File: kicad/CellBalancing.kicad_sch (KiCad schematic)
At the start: 10 parts, among them U15 ETA3000

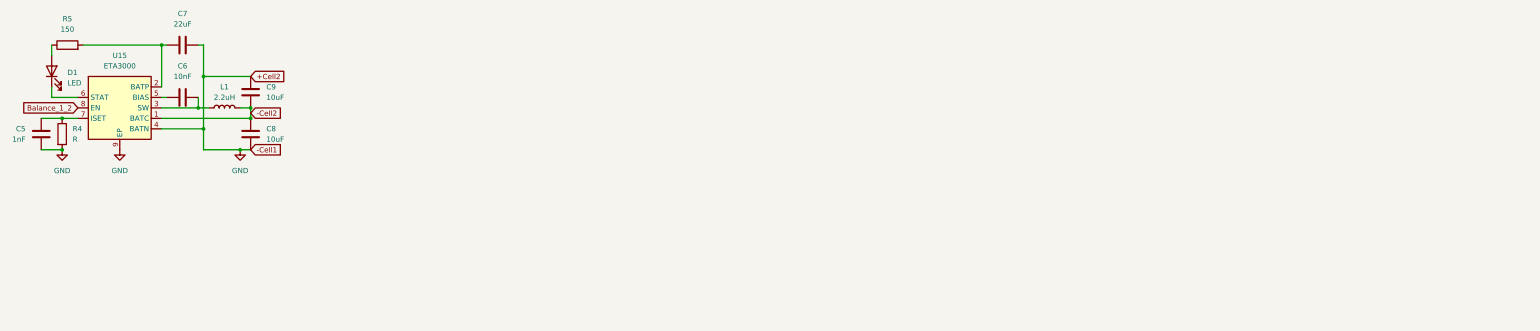
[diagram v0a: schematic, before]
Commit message: .gitignore
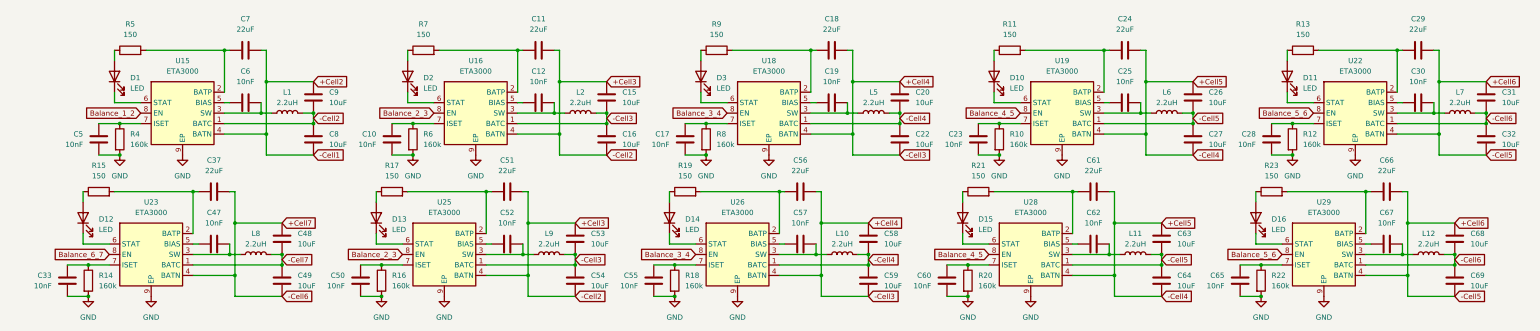
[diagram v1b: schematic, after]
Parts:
- added C10, C12, C17, C19, C23, C25, C28, C30, C33, C47, C50, C52, C55, C57, C60, C62, C65, C67: 10nF, symbol Device:C
- added C11, C18, C24, C29, C37, C51, C56, C61, C66: 22uF, symbol Device:C
- added C15, C16, C20, C22, C26, C27, C31, C32, C48, C49, C53, C54, C58, C59, C63, C64, C68, C69: 10uF, symbol Device:C
- added D10, D11, D12, D13, D14, D15, D16, D2, D3: LED, symbol Device:LED
- added L10, L11, L12, L2, L5, L6, L7, L8, L9: 2.2uH, symbol Device:L
- added R10, R12, R14, R16, R18, R20, R22, R6, R8: 160k, symbol Device:R
- added R11, R13, R15, R17, R19, R21, R23, R7, R9: 150, symbol Device:R
- added U16, U18, U19, U22, U23, U25, U26, U28, U29: ETA3000, Package_DFN_QFN:DFN-8-1EP_2x2mm_P0.5mm_EP0.9x1.3mm, symbol Battery_Management:ETA3000
- C5: value 1nF -> 10nF
- R4: value R -> 160k
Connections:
- net GND: now also C10.2, C17.2, C23.2, C28.2, C33.2, C50.2, C55.2, C60.2, C65.2, R10.2, R12.2, R14.2, R16.2, R18.2, R20.2, R22.2, R6.2, R8.2, U16.9 (EP), U18.9 (EP), U19.9 (EP), U22.9 (EP), U23.9 (EP), U25.9 (EP), U26.9 (EP), U28.9 (EP), U29.9 (EP); no longer C7.2, C8.2, C9.1, U15.4 (BATN)
- net -Cell2 renamed +Cell3
- net +Cell3: now also C11.2, C15.1, C16.2, C51.2, C53.1, C54.2, U16.4 (BATN), U25.4 (BATN)
- new net: D16.2 (A), R23.1
- new net: C66.1, R23.2, U29.2 (BATP)
- new net: C52.1, U25.5 (BIAS)
- new net: C52.2, L9.1, U25.3 (SW)
- new net: C51.1, R17.2, U25.2 (BATP)
- new net: D13.1 (K), U25.6 (STAT)
- new net: C50.1, R16.1, U25.7 (ISET)
- new net: D15.2 (A), R21.1
- new net: C61.1, R21.2, U28.2 (BATP)
- new net: D2.1 (K), U16.6 (STAT)
- new net: D2.2 (A), R7.1
- new net: D16.1 (K), U29.6 (STAT)
- new net: C18.1, R9.2, U18.2 (BATP)
- new net: C19.2, L5.1, U18.3 (SW)
- new net: C19.1, U18.5 (BIAS)
- new net: D3.1 (K), U18.6 (STAT)
- new net: C17.1, R8.1, U18.7 (ISET)
- new net: D15.1 (K), U28.6 (STAT)
- new net: C30.1, U22.5 (BIAS)
- new net: C30.2, L7.1, U22.3 (SW)
- new net: D12.1 (K), U23.6 (STAT)
- new net: D12.2 (A), R15.1
- new net: C65.1, R22.1, U29.7 (ISET)
- new net: C47.1, U23.5 (BIAS)
- new net: C47.2, L8.1, U23.3 (SW)
- new net: C56.1, R19.2, U26.2 (BATP)
- new net: C24.1, R11.2, U19.2 (BATP)
- new net: C60.1, R20.1, U28.7 (ISET)
- new net: C62.2, L11.1, U28.3 (SW)
- new net: C11.1, R7.2, U16.2 (BATP)
- new net: C12.2, L2.1, U16.3 (SW)
- new net: C12.1, U16.5 (BIAS)
- new net: C10.1, R6.1, U16.7 (ISET)
- new net: D14.1 (K), U26.6 (STAT)
- new net: D14.2 (A), R19.1
- new net: C57.2, L10.1, U26.3 (SW)
- new net: D13.2 (A), R17.1
- new net: C33.1, R14.1, U23.7 (ISET)
- new net: D11.1 (K), U22.6 (STAT)
- new net: D11.2 (A), R13.1
- new net: C37.1, R15.2, U23.2 (BATP)
- new net: C67.1, U29.5 (BIAS)
- new net: C67.2, L12.1, U29.3 (SW)
- new net: C29.1, R13.2, U22.2 (BATP)
- new net: C28.1, R12.1, U22.7 (ISET)
- new net: C57.1, U26.5 (BIAS)
- new net: C55.1, R18.1, U26.7 (ISET)
- new net: D3.2 (A), R9.1
- new net: C25.2, L6.1, U19.3 (SW)
- new net: C25.1, U19.5 (BIAS)
- new net: D10.1 (K), U19.6 (STAT)
- new net: C23.1, R10.1, U19.7 (ISET)
- new net: C62.1, U28.5 (BIAS)
- new net: D10.2 (A), R11.1
- new net +Cell2: C7.2, C8.2, C9.1, U15.4 (BATN)
- new net +Cell4: C15.2, C16.1, C18.2, C20.1, C22.2, C53.2, C54.1, C56.2, C58.1, C59.2, L2.2, L9.2, U16.1 (BATC), U18.4 (BATN), U25.1 (BATC), U26.4 (BATN)
- new net +Cell5: C20.2, C22.1, C24.2, C26.1, C27.2, C58.2, C59.1, C61.2, C63.1, C64.2, L10.2, L5.2, U18.1 (BATC), U19.4 (BATN), U26.1 (BATC), U28.4 (BATN)
- new net +Cell6: C26.2, C27.1, C29.2, C31.1, C32.2, C63.2, C64.1, C66.2, C68.1, C69.2, L11.2, L6.2, U19.1 (BATC), U22.4 (BATN), U28.1 (BATC), U29.4 (BATN)
- new net +Cell7: C31.2, C32.1, C37.2, C48.1, C49.2, C68.2, C69.1, L12.2, L7.2, U22.1 (BATC), U23.4 (BATN), U29.1 (BATC)
- new net -Cell7: C48.2, C49.1, L8.2, U23.1 (BATC)
- new net Balance_2_3: U16.8 (EN), U25.8 (EN)
- new net Balance_3_4: U18.8 (EN), U26.8 (EN)
- new net Balance_4_5: U19.8 (EN), U28.8 (EN)
- new net Balance_5_6: U22.8 (EN), U29.8 (EN)
- new net Balance_6_7: U23.8 (EN)
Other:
- moved on the sheet: C5, C6, C7, C8, C9, D1, L1, R4, R5, U15
